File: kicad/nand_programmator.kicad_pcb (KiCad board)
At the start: 2 copper layers, 48 x 41 mm, 42 parts, among them J1 Conn_01x04, J2 Conn_01x03, J3 Conn_02x12_Odd_Even_Left, J4 Conn_02x12_Odd_Even_Right, J5 BOOT0, J6 ~RST, P1 USB, U1 LM1117-3.3, U2 STM32F103VCT6, Y1 Crystal_SMD_8MHz_18pF

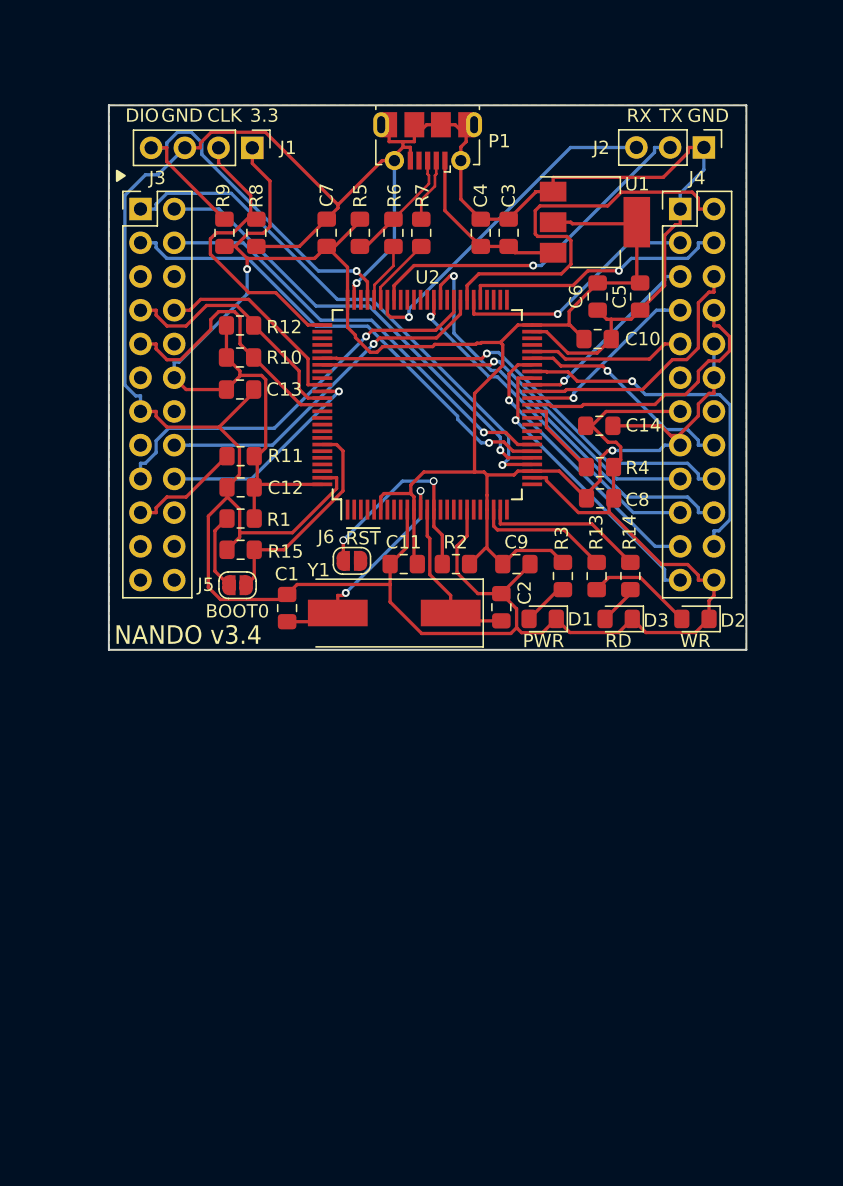
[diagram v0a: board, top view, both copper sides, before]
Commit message: x
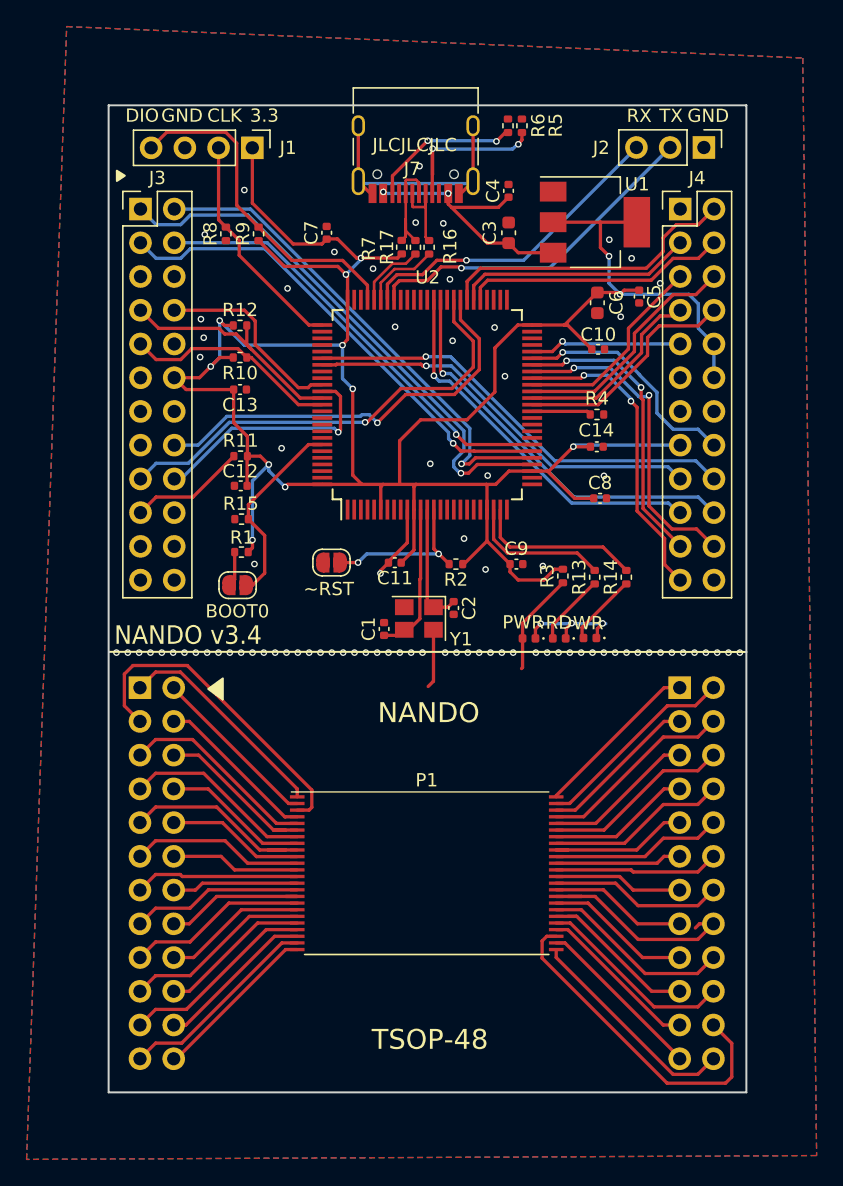
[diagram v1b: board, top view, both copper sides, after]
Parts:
- added J7: USB_C_Receptacle_USB2.0, Connector_USB:USB_C_Receptacle_HRO_TYPE-C-31-M-12, F.Cu at (191.0, 47.2)
- added J8: Conn_02x12_Odd_Even_1, lib_fp:PinSocket_2x12_P2.54mm_Vertical, B.Cu at (170.2, 88.5)
- added J9: Conn_02x12_Odd_Even_2, lib_fp:PinSocket_2x12_P2.54mm_Vertical_2, B.Cu at (210.9, 88.5)
- added R16: 22, Resistor_SMD:R_0402_1005Metric, F.Cu at (192.0, 55.3)
- added R17: 22, Resistor_SMD:R_0402_1005Metric, F.Cu at (191.0, 55.3)
- C1, C10, C11, C12, C13, C14, C2, C4, C5, C7, C8, C9: footprint lib_fp:C_0805_2012Metric_Pad1.15x1.40mm_HandSolder -> Capacitor_SMD:C_0402_1005Metric
- C3, C6: footprint lib_fp:C_0805_2012Metric_Pad1.15x1.40mm_HandSolder -> Capacitor_SMD:C_0603_1608Metric
- D1, D2, D3: footprint lib_fp:LED_0805_2012Metric_Pad1.15x1.40mm_HandSolder -> LED_SMD:LED_0402_1005Metric
- P1: value USB -> TSOP-48; footprint lib_fp:USB_Micro-B_Molex-105017-0001 -> lib_fp:TSOP-I-48_18.4x12mm_P0.5mm
- R1, R10, R11, R12, R13, R14, R15, R2, R3, R4, R8, R9: footprint lib_fp:R_0805_2012Metric_Pad1.15x1.40mm_HandSolder -> Resistor_SMD:R_0402_1005Metric
- R5: value 1.5k -> 5.1k; footprint lib_fp:R_0805_2012Metric_Pad1.15x1.40mm_HandSolder -> Resistor_SMD:R_0402_1005Metric
- R6: value 22 -> 5.1k; footprint lib_fp:R_0805_2012Metric_Pad1.15x1.40mm_HandSolder -> Resistor_SMD:R_0402_1005Metric
- R7: value 22 -> 1.5k; footprint lib_fp:R_0805_2012Metric_Pad1.15x1.40mm_HandSolder -> Resistor_SMD:R_0402_1005Metric
- Y1: value Crystal_SMD_8MHz_18pF -> Crystal_GND24_Small; footprint lib_fp:Crystal_SMD_HC49-SD -> Crystal:Crystal_SMD_3225-4Pin_3.2x2.5mm
- moved P1 55.1 mm to (191.8, 102.5), turned to 0 degrees
- moved R5 14.6 mm to (199.0, 46.2), turned to -90 degrees
- moved R6 11.8 mm to (197.9, 46.2), turned to -90 degrees
- moved D2 10.4 mm to (201.8, 84.8)
- moved C1 7.47 mm to (188.6, 84.1)
- moved R4 3.97 mm to (204.6, 67.9)
- moved C4 3.79 mm to (198.0, 51.1)
- moved C2 3.59 mm to (193.8, 82.5), turned to -90 degrees
- moved D3 2.60 mm to (204.1, 84.7)
- moved R9 2.57 mm to (179.1, 54.3)
- moved R1 2.52 mm to (177.9, 78.3)
- moved R15 2.31 mm to (177.9, 75.8)
- moved R8 2.29 mm to (176.7, 54.3)
- moved Y1 1.90 mm to (191.2, 83.3)
- moved R7 1.82 mm to (189.9, 55.3), turned to -90 degrees
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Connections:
- J3 pad 10: Net-(J3-Pad10) -> unconnected-(J3-Pad10)
- J3 pad 11: Net-(J3-Pad11) -> unconnected-(J3-Pad11)
- J3 pad 14: Net-(J3-Pad14) -> unconnected-(J3-Pad14)
- J3 pad 15: Net-(J3-Pad15) -> unconnected-(J3-Pad15)
- J3 pad 20: Net-(J3-Pad20) -> unconnected-(J3-Pad20)
- J3 pad 21: Net-(J3-Pad21) -> unconnected-(J3-Pad21)
- J3 pad 22: Net-(J3-Pad22) -> unconnected-(J3-Pad22)
- J3 pad 23: Net-(J3-Pad23) -> unconnected-(J3-Pad23)
- J3 pad 24: Net-(J3-Pad24) -> unconnected-(J3-Pad24)
- J3 pad 5: Net-(J3-Pad5) -> unconnected-(J3-Pad5)
- J3 pad 6: Net-(J3-Pad6) -> unconnected-(J3-Pad6)
- J4 pad 35: Net-(J4-Pad35) -> unconnected-(J4-Pad35)
- J4 pad 38: Net-(J4-Pad38) -> unconnected-(J4-Pad38)
- P1 pad 1: +5V -> Net-(J8-Pad1)
- P1 pad 2: /USB_N -> Net-(J8-Pad2)
- P1 pad 3: /USB_P -> Net-(J8-Pad3)
- P1 pad 5: GNDD -> Net-(J8-Pad5)
- P1 pad 6: GNDD -> Net-(J8-Pad6)
- R5 pad 1: /USB_P -> GNDD
- R5 pad 2: +3V3 -> Net-(J7-PadA5)
- R6 pad 1: /USB_DP -> GNDD
- R6 pad 2: /USB_P -> Net-(J7-PadB5)
- R7 pad 1: /USB_DN -> /USB_P
- R7 pad 2: /USB_N -> +3V3
- U2 pad 1: Net-(U2-Pad1) -> unconnected-(U2-Pad1)
- U2 pad 15: Net-(U2-Pad15) -> unconnected-(U2-Pad15)
- U2 pad 16: Net-(U2-Pad16) -> unconnected-(U2-Pad16)
- U2 pad 17: Net-(U2-Pad17) -> unconnected-(U2-Pad17)
- U2 pad 18: Net-(U2-Pad18) -> unconnected-(U2-Pad18)
- U2 pad 2: Net-(U2-Pad2) -> unconnected-(U2-Pad2)
- U2 pad 20: Net-(U2-Pad20) -> unconnected-(U2-Pad20)
- U2 pad 21: Net-(U2-Pad21) -> unconnected-(U2-Pad21)
- U2 pad 25: Net-(U2-Pad25) -> unconnected-(U2-Pad25)
- U2 pad 26: Net-(U2-Pad26) -> unconnected-(U2-Pad26)
- U2 pad 3: Net-(U2-Pad3) -> unconnected-(U2-Pad3)
- U2 pad 33: Net-(U2-Pad33) -> unconnected-(U2-Pad33)
- U2 pad 34: Net-(U2-Pad34) -> unconnected-(U2-Pad34)
- U2 pad 35: Net-(U2-Pad35) -> unconnected-(U2-Pad35)
- U2 pad 36: Net-(U2-Pad36) -> unconnected-(U2-Pad36)
- U2 pad 4: Net-(U2-Pad4) -> unconnected-(U2-Pad4)
- U2 pad 47: Net-(U2-Pad47) -> unconnected-(U2-Pad47)
- U2 pad 48: Net-(U2-Pad48) -> unconnected-(U2-Pad48)
- U2 pad 5: Net-(U2-Pad5) -> unconnected-(U2-Pad5)
- U2 pad 51: Net-(U2-Pad51) -> unconnected-(U2-Pad51)
- U2 pad 52: Net-(U2-Pad52) -> unconnected-(U2-Pad52)
- U2 pad 53: Net-(U2-Pad53) -> unconnected-(U2-Pad53)
- U2 pad 54: Net-(U2-Pad54) -> unconnected-(U2-Pad54)
- U2 pad 60: Net-(U2-Pad60) -> unconnected-(U2-Pad60)
- U2 pad 63: Net-(U2-Pad63) -> unconnected-(U2-Pad63)
- U2 pad 64: Net-(U2-Pad64) -> unconnected-(U2-Pad64)
- U2 pad 65: Net-(U2-Pad65) -> unconnected-(U2-Pad65)
- U2 pad 66: Net-(U2-Pad66) -> unconnected-(U2-Pad66)
- U2 pad 67: Net-(U2-Pad67) -> unconnected-(U2-Pad67)
- U2 pad 7: Net-(U2-Pad7) -> unconnected-(U2-Pad7)
- U2 pad 73: Net-(U2-Pad73) -> unconnected-(U2-Pad73)
- U2 pad 77: Net-(U2-Pad77) -> unconnected-(U2-Pad77)
- U2 pad 78: Net-(U2-Pad78) -> unconnected-(U2-Pad78)
- U2 pad 79: Net-(U2-Pad79) -> unconnected-(U2-Pad79)
- U2 pad 8: Net-(U2-Pad8) -> unconnected-(U2-Pad8)
- U2 pad 80: Net-(U2-Pad80) -> unconnected-(U2-Pad80)
- U2 pad 83: Net-(U2-Pad83) -> unconnected-(U2-Pad83)
- U2 pad 84: Net-(U2-Pad84) -> unconnected-(U2-Pad84)
- U2 pad 89: Net-(U2-Pad89) -> unconnected-(U2-Pad89)
- U2 pad 9: Net-(U2-Pad9) -> unconnected-(U2-Pad9)
- U2 pad 90: Net-(U2-Pad90) -> unconnected-(U2-Pad90)
- U2 pad 91: Net-(U2-Pad91) -> unconnected-(U2-Pad91)
- U2 pad 92: Net-(U2-Pad92) -> unconnected-(U2-Pad92)
- U2 pad 93: Net-(U2-Pad93) -> unconnected-(U2-Pad93)
- U2 pad 95: Net-(U2-Pad95) -> unconnected-(U2-Pad95)
- U2 pad 96: Net-(U2-Pad96) -> unconnected-(U2-Pad96)
- U2 pad 97: Net-(U2-Pad97) -> unconnected-(U2-Pad97)
- U2 pad 98: Net-(U2-Pad98) -> unconnected-(U2-Pad98)
- Y1 pad 2: Net-(C1-Pad1) -> GNDD
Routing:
- net GNDD: track 270.6 -> 38.0 mm, vias 1 -> 32
- net Net-(J9-Pad27): track 0.00 -> 25.4 mm
- net Net-(J8-Pad3): track 0.00 -> 24.8 mm
- net +3V3: track 179.4 -> 202.2 mm, vias 2 -> 12
- net Net-(J8-Pad1): track 0.00 -> 16.6 mm
- net Net-(J9-Pad25): track 0.00 -> 16.6 mm
- net Net-(J9-Pad33): track 0.00 -> 16.2 mm
- net Net-(J8-Pad23): track 0.00 -> 15.5 mm
- net Net-(J9-Pad47): track 0.00 -> 15.5 mm
- net Net-(J8-Pad9): track 0.00 -> 15.0 mm
- net Net-(J9-Pad29): track 0.00 -> 14.9 mm
- net Net-(J8-Pad5): track 0.00 -> 14.9 mm
- net Net-(J8-Pad21): track 0.00 -> 14.8 mm
- net Net-(J9-Pad45): track 0.00 -> 14.8 mm
- net Net-(J9-Pad31): track 0.00 -> 14.3 mm
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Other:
- board size 48 x 41 mm -> 48 x 74.3 mm
- net class Default removed
- net class VDD removed
- rule pad_to_mask_clearance: 0.2 -> 0
- board text added: "JLCJLCJLC"
- board text added: "NANDO"
- board text added: "TSOP-48"
